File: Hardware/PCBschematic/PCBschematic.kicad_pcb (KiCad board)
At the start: 2 copper layers, 85 x 65 mm, 49 parts, among them J3 Conn_01x02, J4 Conn_02x07_Odd_Even, J5 Conn_01x02, J6 Conn_01x02, J7 Conn_01x02, J8 batterie, J9 Conn_01x08, Q1 SQ2310ES, Q2 SQ2310ES, Q3 SQ2310ES, Q4 SQ2310ES, SW1 SW_Push, SW2 SW_Push, U1 STM32L412KBTx, U2 NCS210, U3 NCS210, U4 NCS210, U5 NCS210, U6 regulator_17395xx36

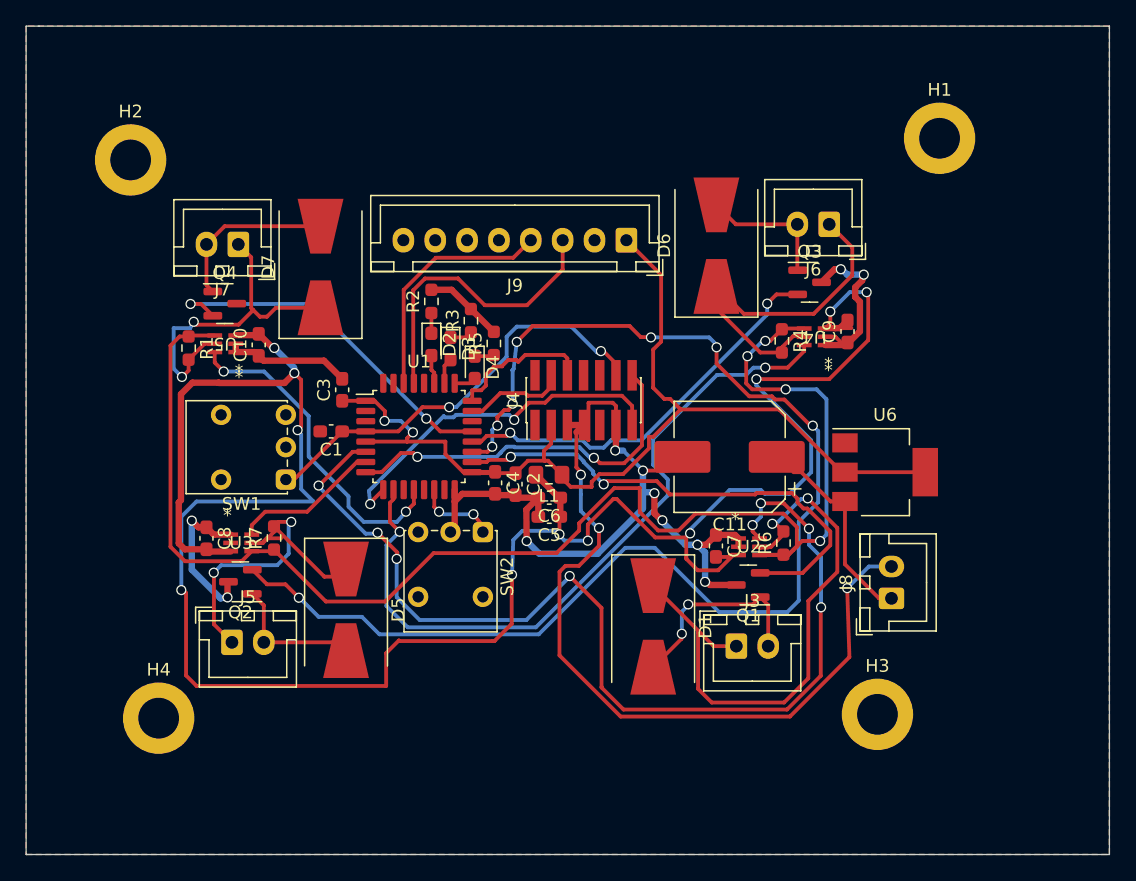
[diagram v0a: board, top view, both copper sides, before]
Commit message: pcb_mise_en_place_okay_reste_3_erreurs git commit -m pcb_mise_en_place_okay_reste_3_erreurs
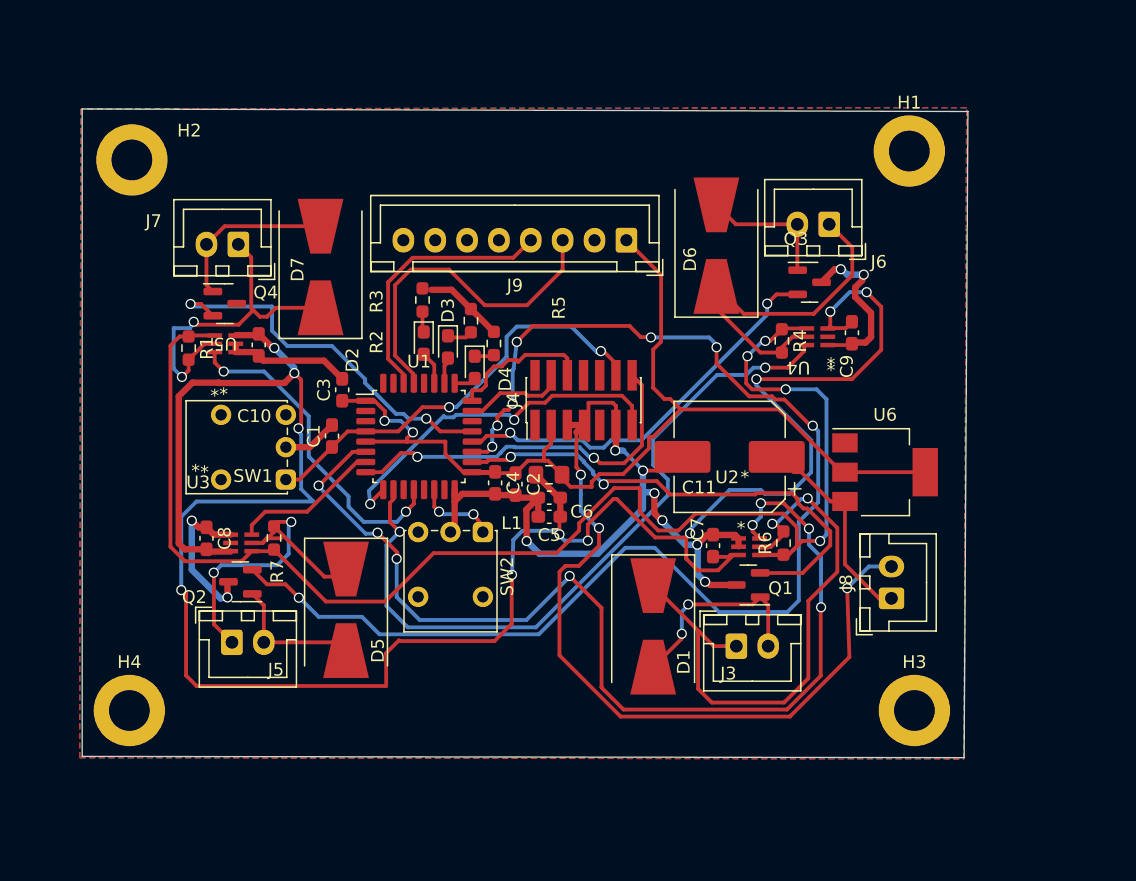
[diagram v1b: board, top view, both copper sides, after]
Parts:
- moved H3 2.92 mm to (188.7, 138.7)
- moved H1 2.58 mm to (188.3, 94.8)
- moved H4 2.38 mm to (127.1, 138.7)
- moved R2 0.71 mm to (150.1, 106.5)
- moved D2 0.61 mm to (150.2, 109.9)
- moved C1 0.37 mm to (143.0, 117.2), turned to 90 degrees
- moved C9 0.36 mm to (183.8, 109.1)
- moved D3 0.24 mm to (152.1, 110.2)
- moved C7 0.23 mm to (172.9, 125.8)
- moved U4 0.20 mm to (181.1, 109.4)
- moved H2 0.10 mm to (127.3, 95.5)
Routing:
- net GND: track 162.8 -> 167.0 mm
- net I2C_SCL: track 23.7 -> 26.5 mm
- net I2C_SDA: track 18.9 -> 21.0 mm
- net PWM_4: track 28.6 -> 29.9 mm
- net +3.3VA: track 177.6 -> 178.3 mm
- net Reset_Buton : track 32.7 -> 33.3 mm
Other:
- board size 85 x 65 mm -> 69.5 x 50.9 mm
